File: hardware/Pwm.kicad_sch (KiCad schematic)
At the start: 69 parts, among them J10 Conn_01x03_Male, J11 Conn_01x03_Male, J12 Conn_01x03_Male, J13 Conn_01x03_Male, J14 Conn_01x03_Male, J15 Conn_01x03_Male, J16 JST XH, J17 KF350, J18 JST XH, J19 JST XH, J20 KF350, J21 JST XH, J4 JST XH, J5 KF129, J6 KF350, J7 Conn_01x03_Male, J8 Conn_01x03_Male, J9 Conn_01x03_Male, U6 74HCT04

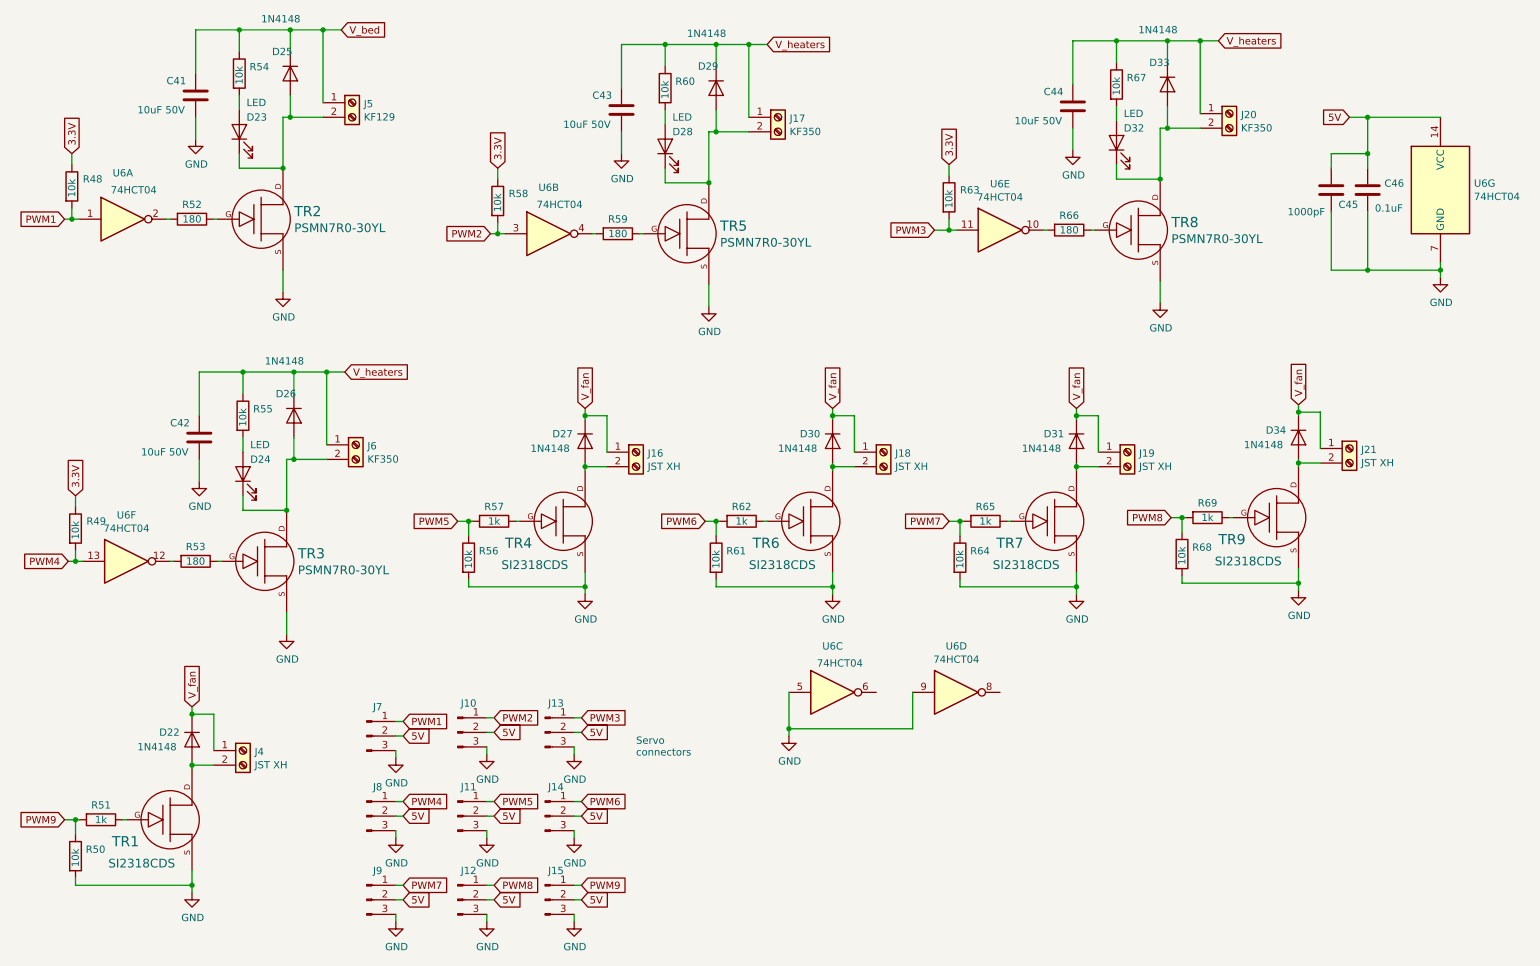
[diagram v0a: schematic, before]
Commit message: Update PrntrBoard fabrication files.
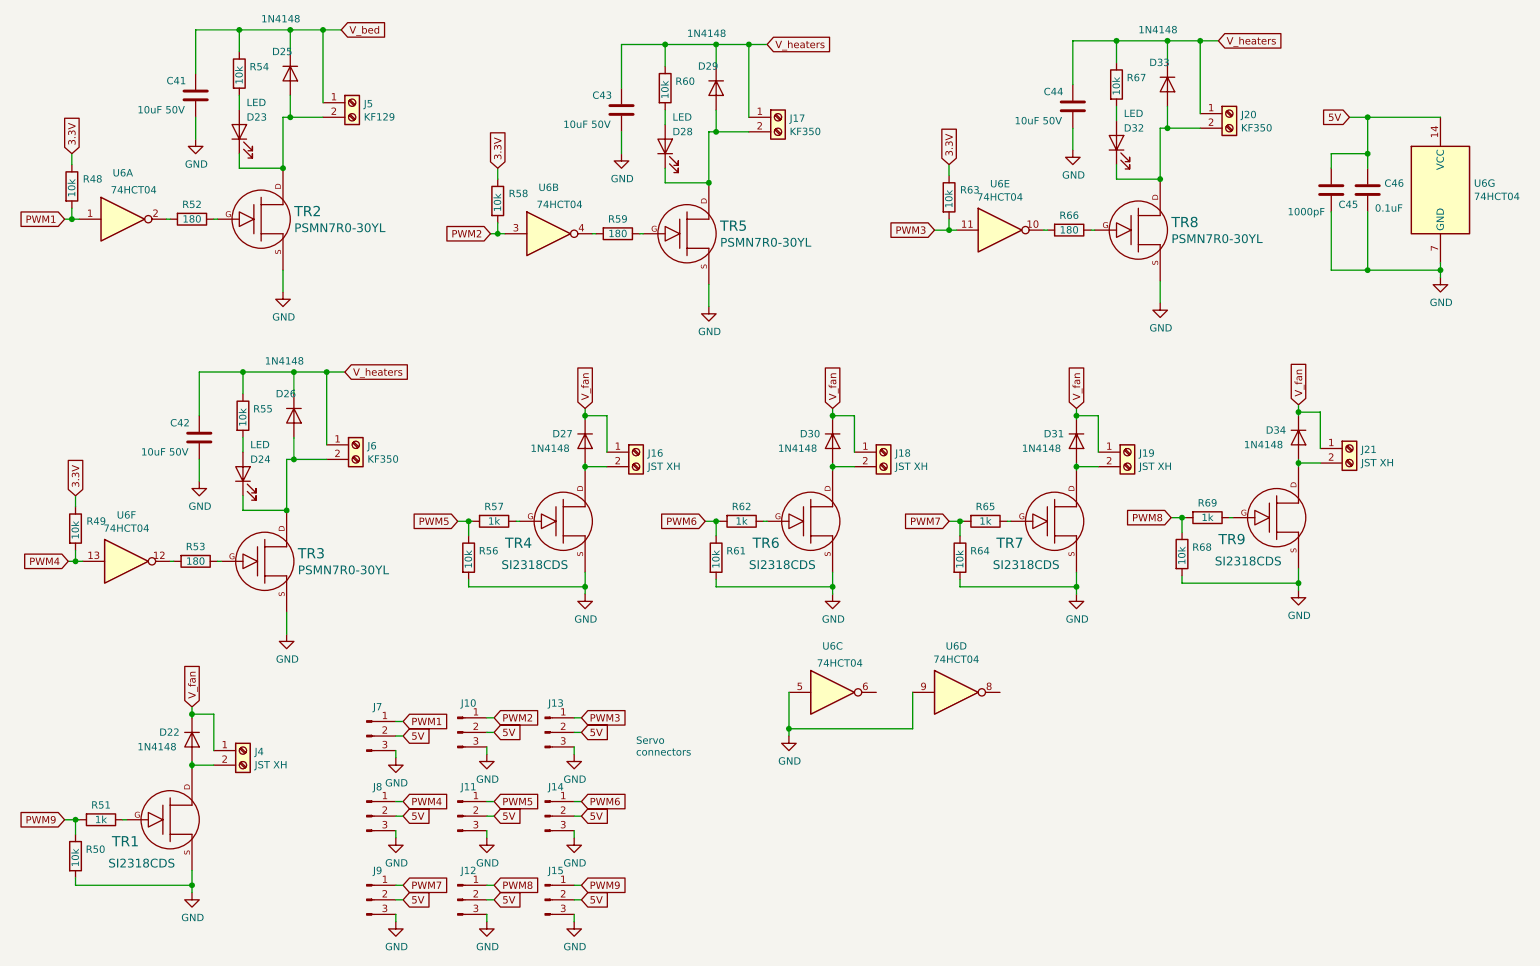
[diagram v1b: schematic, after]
